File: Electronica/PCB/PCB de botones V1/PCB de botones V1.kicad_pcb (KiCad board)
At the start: 2 copper layers, 80.3 x 28.4 mm, 14 parts, among them J2 Conn_02x05_Counter_Clockwise, SW2 SW_Push, SW4 SW_Push, SW9 SW_SPST

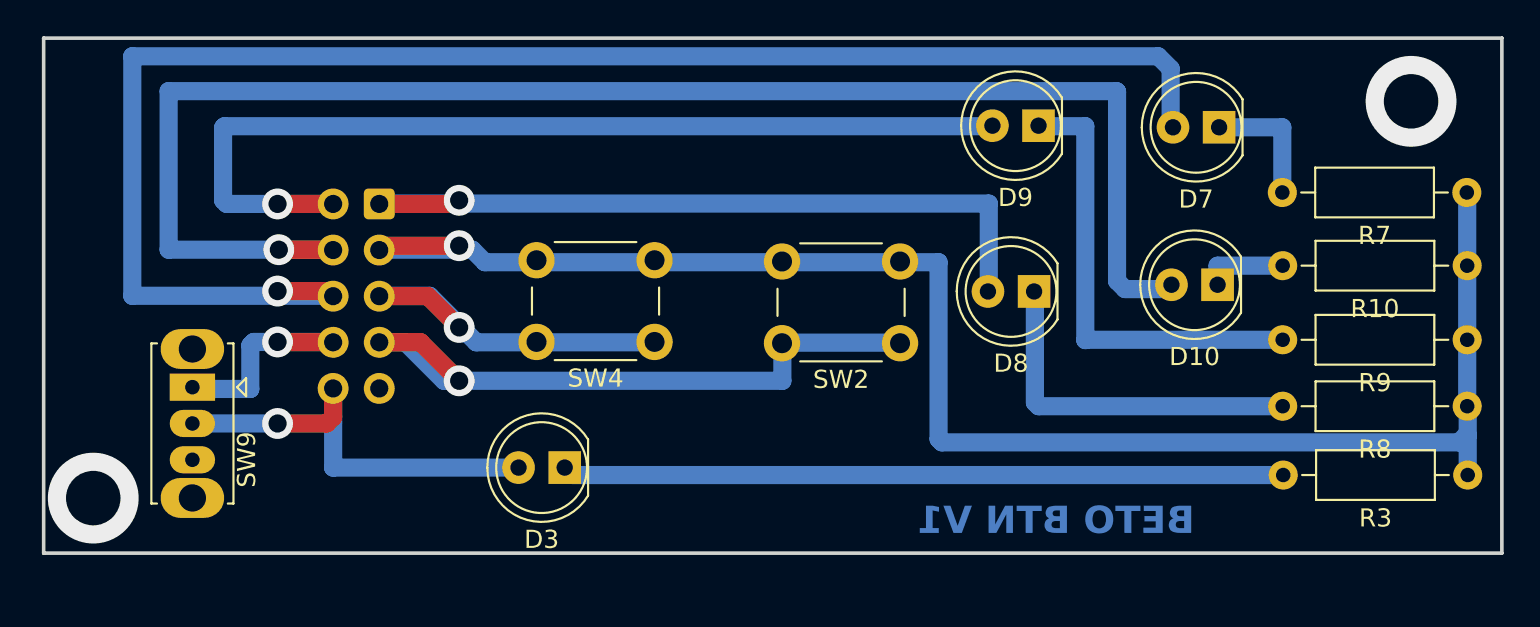
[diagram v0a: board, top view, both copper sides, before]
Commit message: ?
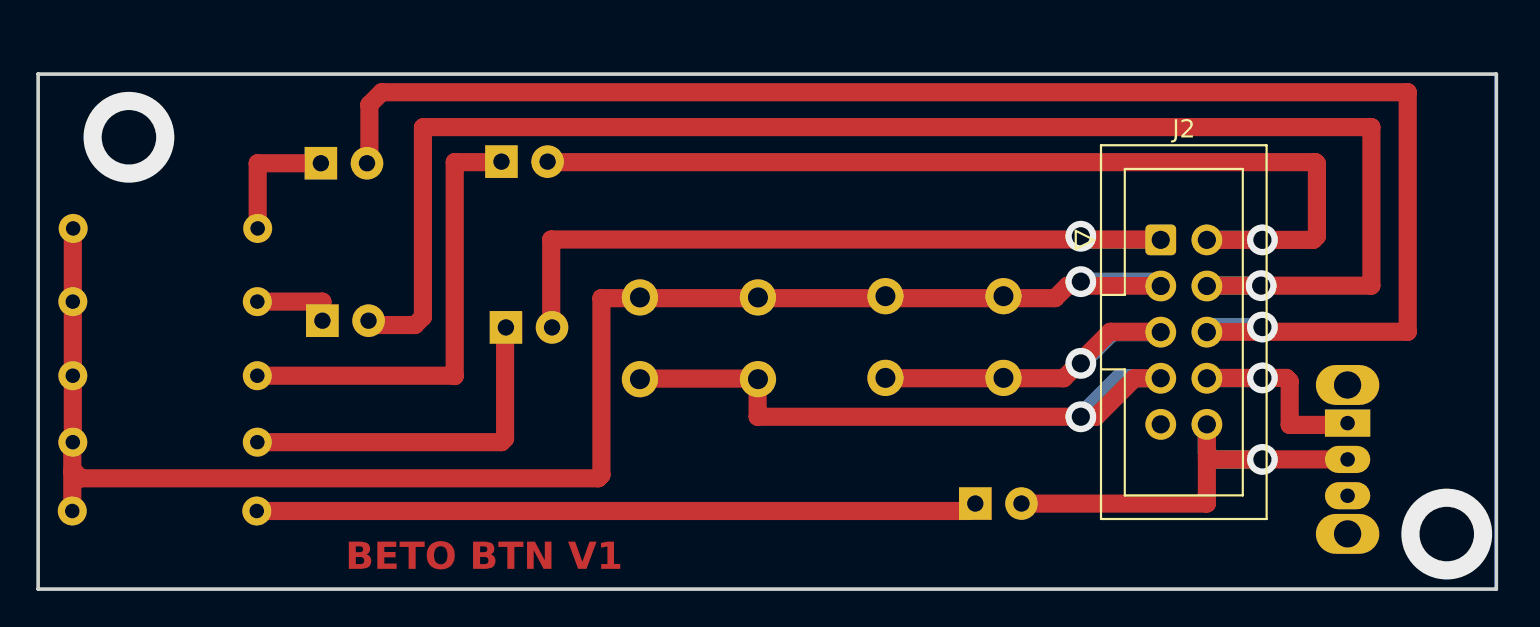
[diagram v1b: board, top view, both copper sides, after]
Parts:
- D10, D3, D7, D8, D9, R10, R3, R7, R8, R9, SW2, SW4, SW9: moved to B.Cu
- J2: moved to F.Cu
- moved R3 76.9 mm to (151.2, 98.6), turned to 0 degrees
- moved R10 76.8 mm to (151.2, 87.1), turned to 0 degrees
- moved R8 76.8 mm to (151.2, 94.8), turned to 0 degrees
- moved R9 76.8 mm to (151.2, 91.2), turned to 0 degrees
- moved R7 76.8 mm to (151.2, 83.0), turned to 0 degrees
- moved SW9 63.6 mm to (221.4, 93.8)
- moved D7 49.5 mm to (164.9, 79.5), turned to 0 degrees
- moved D10 49.3 mm to (165.0, 88.1), turned to 0 degrees
- moved J2 43.1 mm to (211.1, 83.7), turned to 0 degrees
- moved D9 29.6 mm to (174.8, 79.4), turned to 0 degrees
- moved D8 29.2 mm to (175.1, 88.5), turned to 0 degrees
- moved D3 22.7 mm to (200.9, 98.2), turned to 0 degrees
- moved SW2 14.5 mm to (182.5, 91.3), turned to 0 degrees
- moved SW4 12.9 mm to (196.0, 91.3), turned to 0 degrees
